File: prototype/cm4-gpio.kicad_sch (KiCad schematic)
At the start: 2 parts, among them J2 USB4105-GF-A

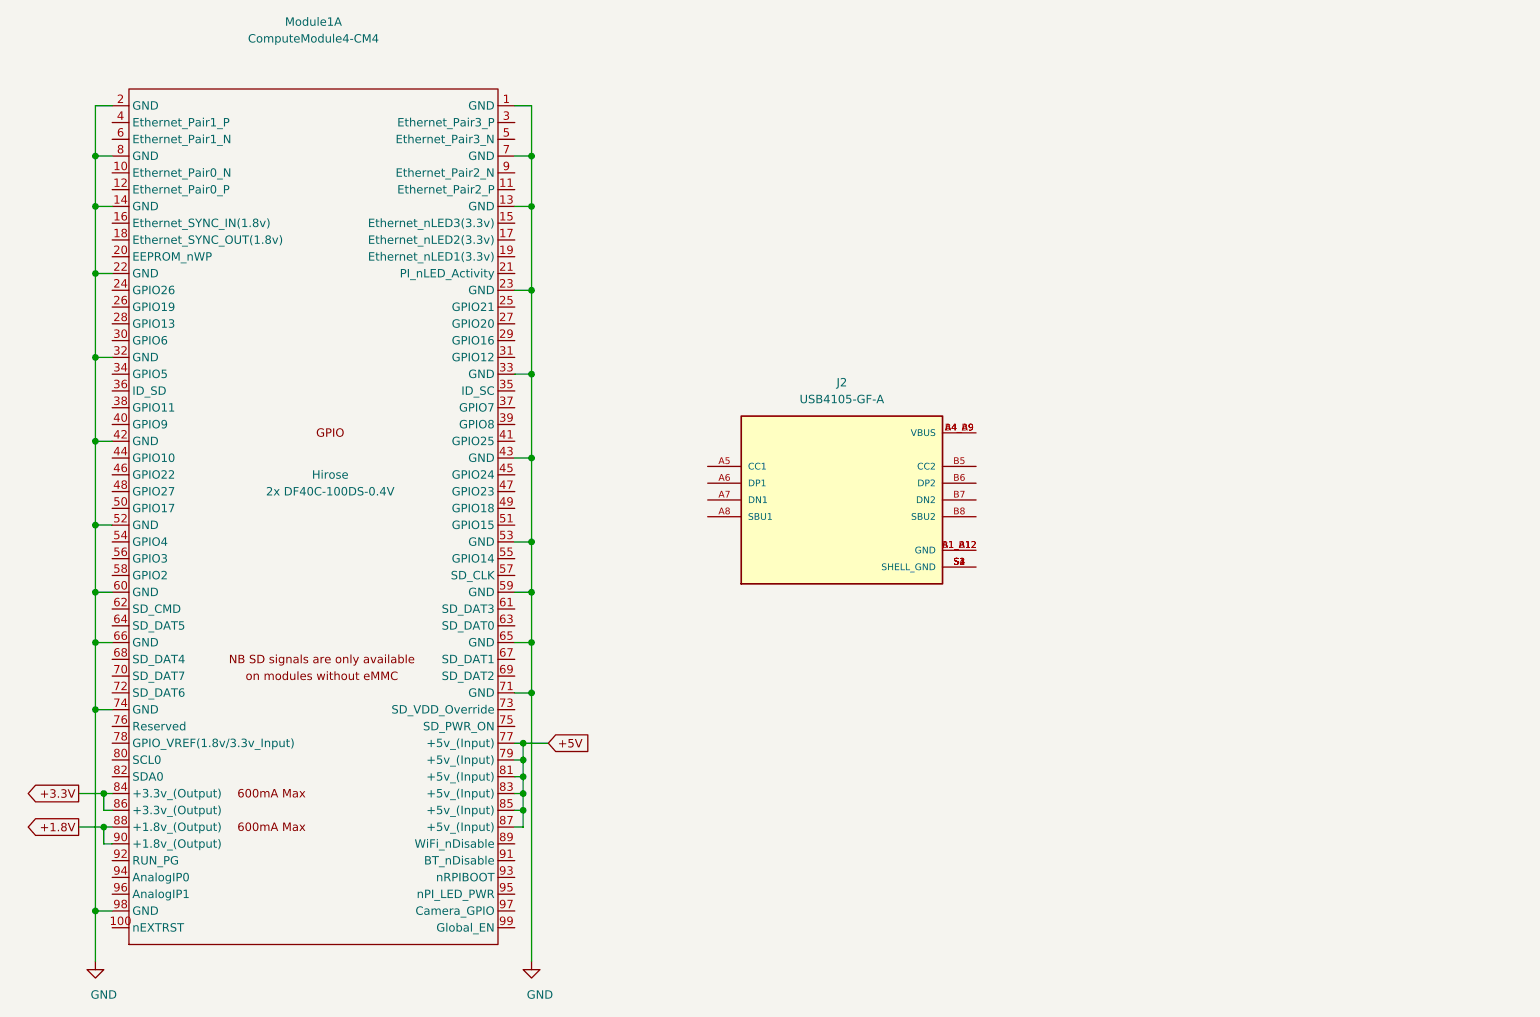
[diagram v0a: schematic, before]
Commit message: update
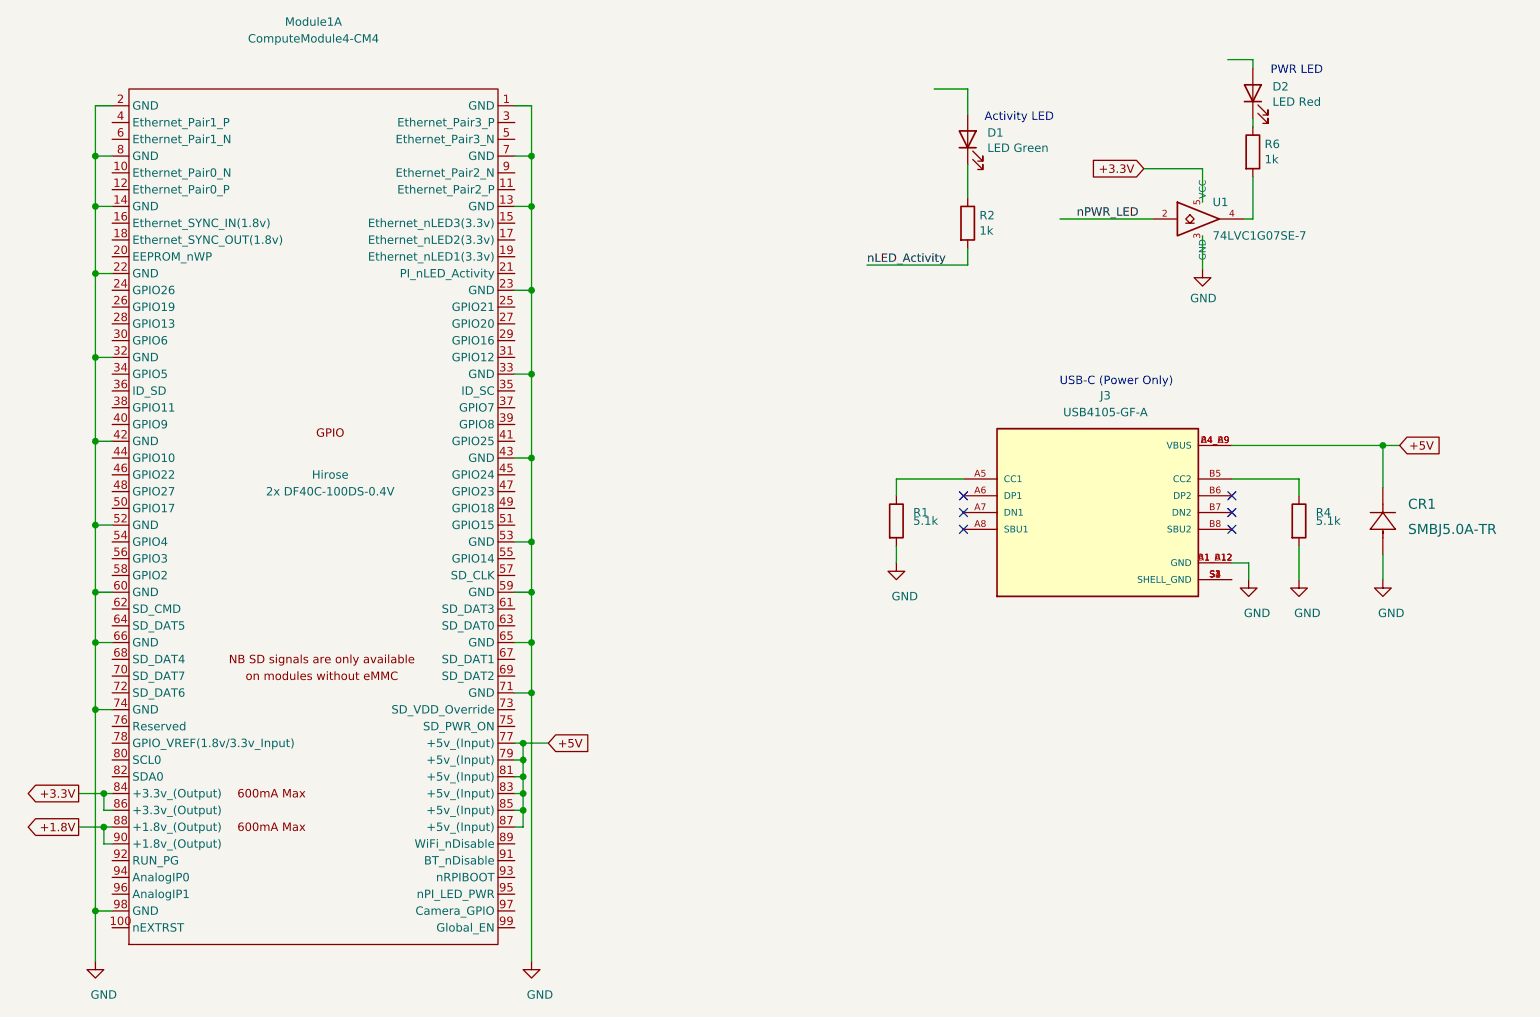
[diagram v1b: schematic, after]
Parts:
- removed J2: USB4105-GF-A, GCT_USB4105-GF-A, symbol USB4105-GF-A:USB4105-GF-A
- added CR1: SMBJ5.0A-TR, footprints:SMBJ5.0A-TR, symbol 2020-11-06_22-01-36:SMBJ5.0A-TR
- added D1: LED Green, LED_SMD:LED_0603_1608Metric, symbol Device:LED
- added D2: LED Red, LED_SMD:LED_0603_1608Metric, symbol Device:LED
- added J3: USB4105-GF-A, USB4105-GF-A:GCT_USB4105-GF-A, symbol USB4105-GF-A:USB4105-GF-A
- added R1, R4: 5.1k, Resistor_SMD:R_0603_1608Metric_Pad0.98x0.95mm_HandSolder, symbol Device:R
- added R2, R6: 1k, Resistor_SMD:R_0603_1608Metric_Pad0.98x0.95mm_HandSolder, symbol Device:R
- added U1: 74LVC1G07SE-7, Package_TO_SOT_SMD:SOT-353_SC-70-5, symbol CM4IO:74LVC1G07_copy
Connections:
- net +3.3V: now also U1.5 (VCC)
- net +5V: now also CR1.1, J3.A4_B9 (VBUS), J3.B4_A9 (VBUS)
- net GND: now also CR1.2, J3.A1_B12 (GND), J3.B1_A12 (GND), R1.2, R4.2, U1.3 (GND)
- new net: D2.1 (K), R6.1
- new net: J3.A5 (CC1), R1.1
- new net: J3.B5 (CC2), R4.1
- new net: J3.S1 (SHELL_GND), J3.S2 (SHELL_GND), J3.S3 (SHELL_GND), J3.S4 (SHELL_GND)
- new net: R6.2, U1.4
- new net: D1.1 (K), R2.1
- new net nLED_Activity: R2.2
- new net nPWR_LED: U1.2
- no-connect marks 0 -> 6
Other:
- note added: "Activity LED"
- note added: "PWR LED"
- note added: "USB-C (Power Only)"
